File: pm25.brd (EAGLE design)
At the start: 55.9 x 33 mm, 39 parts, among them J1 CON-0024, Q1 TR-0001, Q2 TR-0001, Q3 TR-0003, U1 POWER-VREG-FB-EN-SW-350MA, U2 CCS811B-JOPD500, U3 POWER-SWITCH-SIP32509DT, U4 SI7021-A20-GM1R

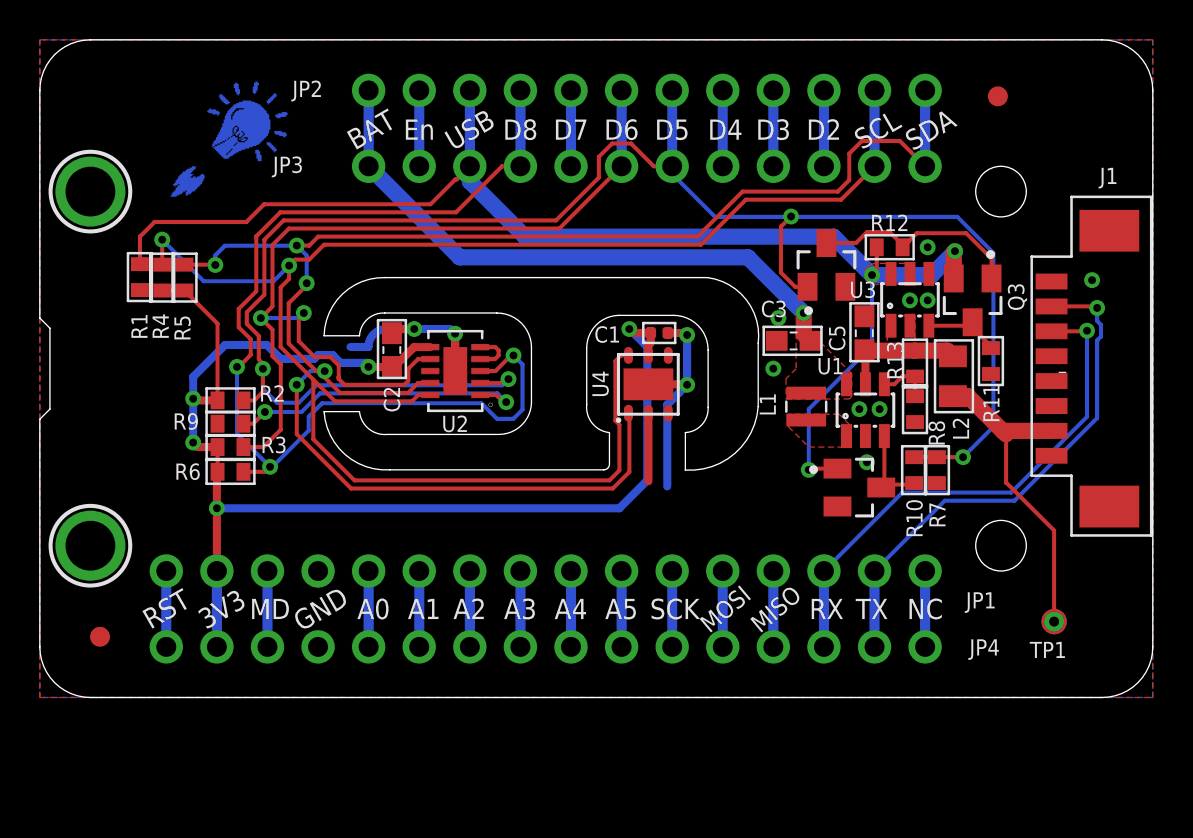
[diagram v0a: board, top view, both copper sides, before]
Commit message: Version 5!
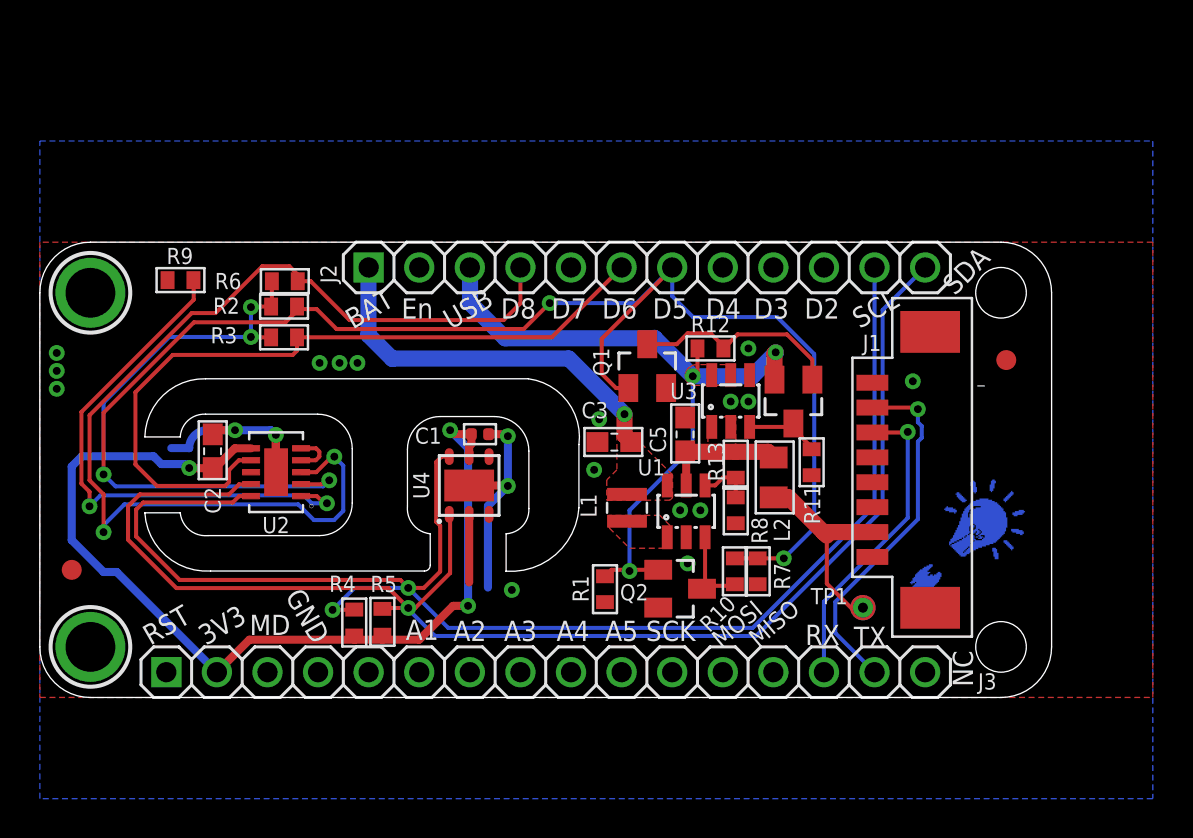
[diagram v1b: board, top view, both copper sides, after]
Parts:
- removed JP1, JP4: (no value), microbuilder:1X16_ROUND
- removed JP2, JP3: (no value), microbuilder:1X12_ROUND
- added J2: HEADER-12, wolff-den:CON-HEADER-1X12
- added J3: HEADER-16, wolff-den:CON-HEADER-1X16
- U3: value POWER-SWITCH-SIP32509DT -> POWER-SWITCH-SIP32508-SO23-6
- moved U$1 42.0 mm to (43.4, 4.82)
- moved R1 28.1 mm to (28.4, 5.44)
- moved R5 19.9 mm to (17.2, 3.80)
- moved R4 19.8 mm to (15.8, 3.76)
- moved U$35 13.2 mm to (48.5, 16.9)
- moved C1 10.3 mm to (22.1, 13.2)
- moved C2 10.3 mm to (8.68, 12.4)
- moved C5 10.3 mm to (32.4, 13.2)
- moved J1 10.3 mm to (41.8, 11.4)
- moved L1 10.3 mm to (29.5, 9.53)
- moved L2 10.3 mm to (36.8, 11.0)
- moved Q1 10.3 mm to (30.5, 16.6)
- moved Q2 10.3 mm to (32.1, 5.46)
- moved Q3 10.3 mm to (37.8, 14.9)
- moved R10 10.3 mm to (34.9, 6.33)
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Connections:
- net !RESET: now also J3.1; no longer JP1.16, JP4.16
- net +3V3: now also J3.2; no longer JP1.15, JP4.15
- net A0: now also J3.5; no longer JP1.12, JP4.12
- net A1: now also J3.6; no longer JP1.11, JP4.11
- net A2: now also J3.7; no longer JP1.10, JP4.10
- net A3: now also J3.8; no longer JP1.9, JP4.9
- net A4: now also J3.9; no longer JP1.8, JP4.8
- net A5: now also J3.10; no longer JP1.7, JP4.7
- net D2: now also J2.10; no longer JP2.10, JP3.10
- net D3: now also J2.9; no longer JP2.9, JP3.9
- net D4: now also J2.8; no longer JP2.8, JP3.8
- net D5: now also J2.7; no longer JP2.7, JP3.7
- net D6: now also J2.6; no longer JP2.6, JP3.6
- net D7: now also J2.5; no longer JP2.5, JP3.5
- net D8: now also J2.4; no longer JP2.4, JP3.4
- net EN: now also J2.2; no longer JP2.2, JP3.2
- net GND: now also J3.4; no longer JP1.13, JP4.13
- net MD: now also J3.3; no longer JP1.14, JP4.14
- net MISO: now also J3.13; no longer JP1.4, JP4.4
- net MOSI: now also J3.12; no longer JP1.5, JP4.5
- net NC: now also J3.16; no longer JP1.1, JP4.1
- net RX: now also J3.14; no longer JP1.3, JP4.3
- net SCK: now also J3.11; no longer JP1.6, JP4.6
- net SCL: now also J2.11; no longer JP2.11, JP3.11
- net SDA: now also J2.12; no longer JP2.12, JP3.12
- net TX: now also J3.15; no longer JP1.2, JP4.2
- net VBAT: now also J2.1; no longer JP2.1, JP3.1
- net VBUS: now also J2.3; no longer JP2.3, JP3.3
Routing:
- net VBUS: track 66.2 -> 36.2 mm
- net SDA: track 84.5 -> 71.3 mm, vias 5 -> 1
- net N$4: track 15.5 -> 27.6 mm
- net VBAT: track 30.2 -> 19.4 mm
- net RX: track 26.3 -> 15.6 mm
- net D6: track 47.7 -> 38.2 mm, vias 2 -> 0
- net SCL: track 82.9 -> 74.5 mm
- net D5: track 88.7 -> 80.7 mm
- net TX: track 26.2 -> 18.2 mm
- net V5V0_HAT: track 16.3 -> 10.9 mm
- net SCK: track 3.81 -> 0.00 mm
- net NC: track 3.81 -> 0.00 mm
- net MOSI: track 3.81 -> 0.00 mm
- net MISO: track 3.81 -> 0.00 mm
- net MD: track 3.81 -> 0.00 mm
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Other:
- board size 55.9 x 33 mm -> 50.8 x 22.9 mm
- board text added: "BRD-0010-05"
- board text added: "CCS811"
- board text added: "Si7021"
- board text removed: "BRD-0010-04"
